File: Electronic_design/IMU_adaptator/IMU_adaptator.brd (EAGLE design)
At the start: 47.7 x 34.1 mm, 8 parts, among them J1 CLM-110-02-XX-D

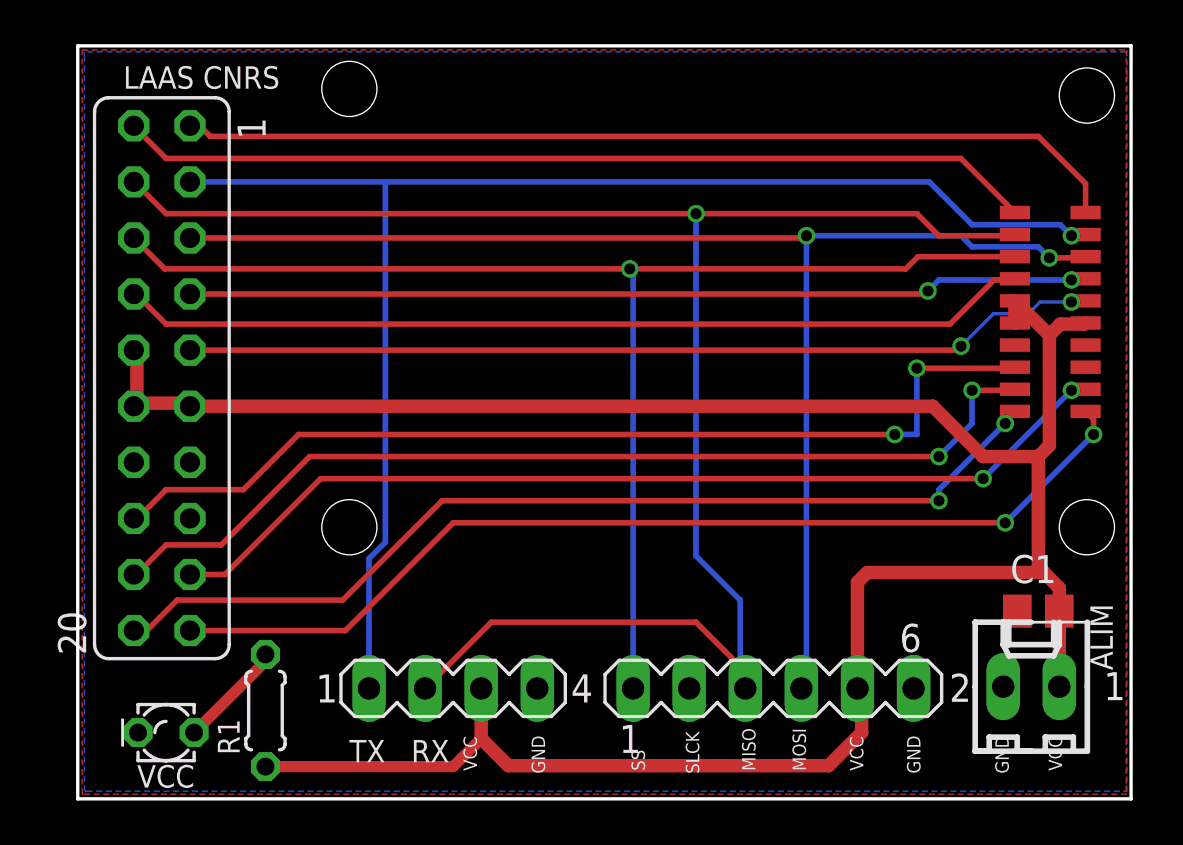
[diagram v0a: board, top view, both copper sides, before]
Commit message: nouveau routage
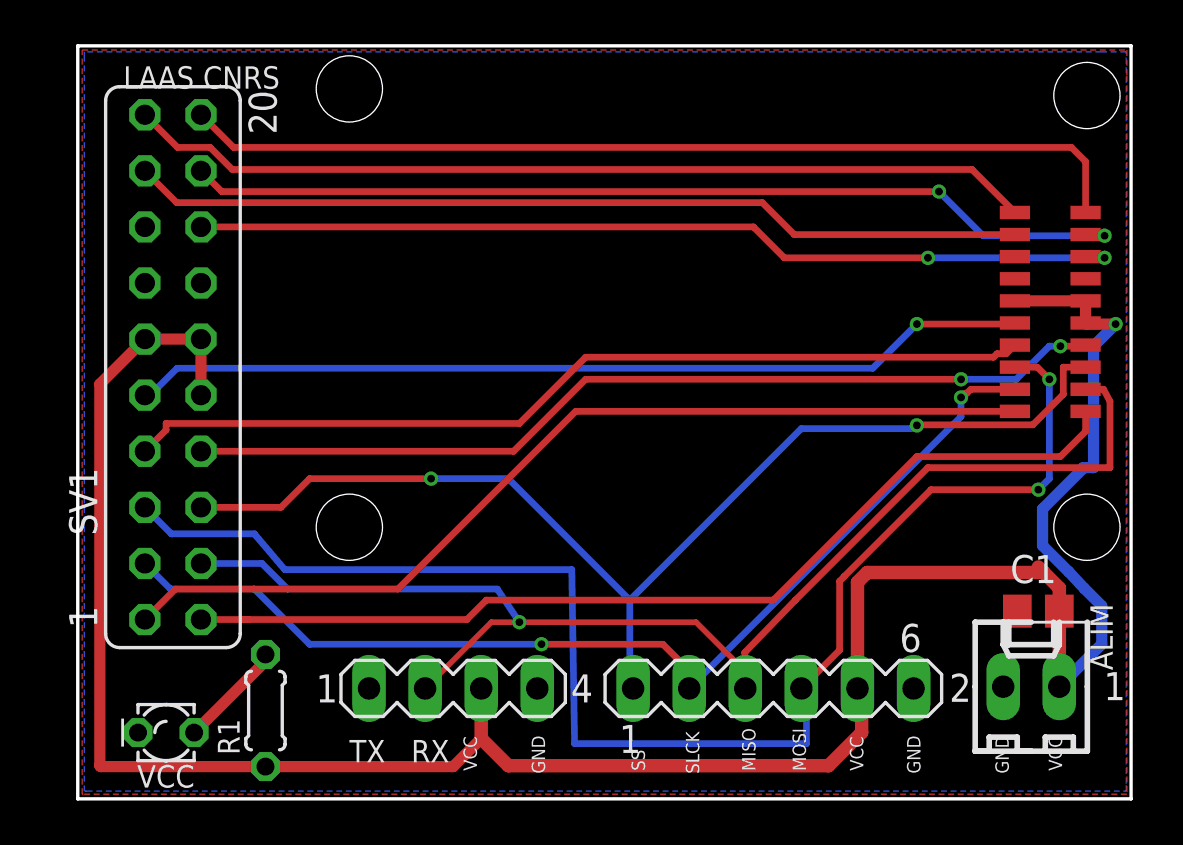
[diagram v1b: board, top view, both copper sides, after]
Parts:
- moved SV1 0.71 mm to (4.31, 19.6), turned to 90 degrees
- turned J1 to 90 degrees
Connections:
- net N$1 renamed 1
- net N$2 renamed 2
- net N$20 renamed 20
- net SCK/TX: now also J1.3, SV1.3
- net SLCK/TX: no longer J1.3, SV1.3
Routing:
- net SLCK/TX: track 65.0 -> 0.00 mm, vias 1 -> 0
- net SCK/TX: track 0.00 -> 48.3 mm, vias 0 -> 2
- net MISO/RX: track 81.1 -> 59.2 mm
- net SS: track 59.8 -> 52.1 mm, vias 1 -> 2
- net N$14: track 45.8 -> 41.2 mm, vias 2 -> 0
- net N$13: track 44.0 -> 40.6 mm, vias 2 -> 0
- net MOSI: track 61.6 -> 64.8 mm
- net 2: track 41.5 -> 44.7 mm
- net N$23: track 44.5 -> 42.4 mm
- net VCC: track 113.6 -> 112.3 mm, vias 0 -> 1
- net N$22: track 44.3 -> 43.0 mm
- net 20: track 44.4 -> 43.2 mm, vias 2 -> 0
- net N$18: track 41.3 -> 42.1 mm, vias 0 -> 2
- net N$9: track 41.5 -> 40.8 mm, vias 2 -> 1
- net N$8: track 40.8 -> 41.6 mm, vias 2 -> 0
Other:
- board text removed: "2"
- board text removed: "3"
- board text removed: "4"
